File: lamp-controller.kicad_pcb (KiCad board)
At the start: 2 copper layers, 34.9 x 26.5 mm, 33 parts, among them J1 Conn_01x02_Pin, J2 Conn_ARM_JTAG_SWD_10, J3 Conn_01x04_Socket, J4 Conn_01x03_Socket, J5 Conn_01x03_Male, Q1 DMN2053UVT, Q2 DMN2053UVT, SW1 SW_SPST, SW2 SW_Push, U1 MIC5365-3.3YC5, U2 STM32L010F4Px

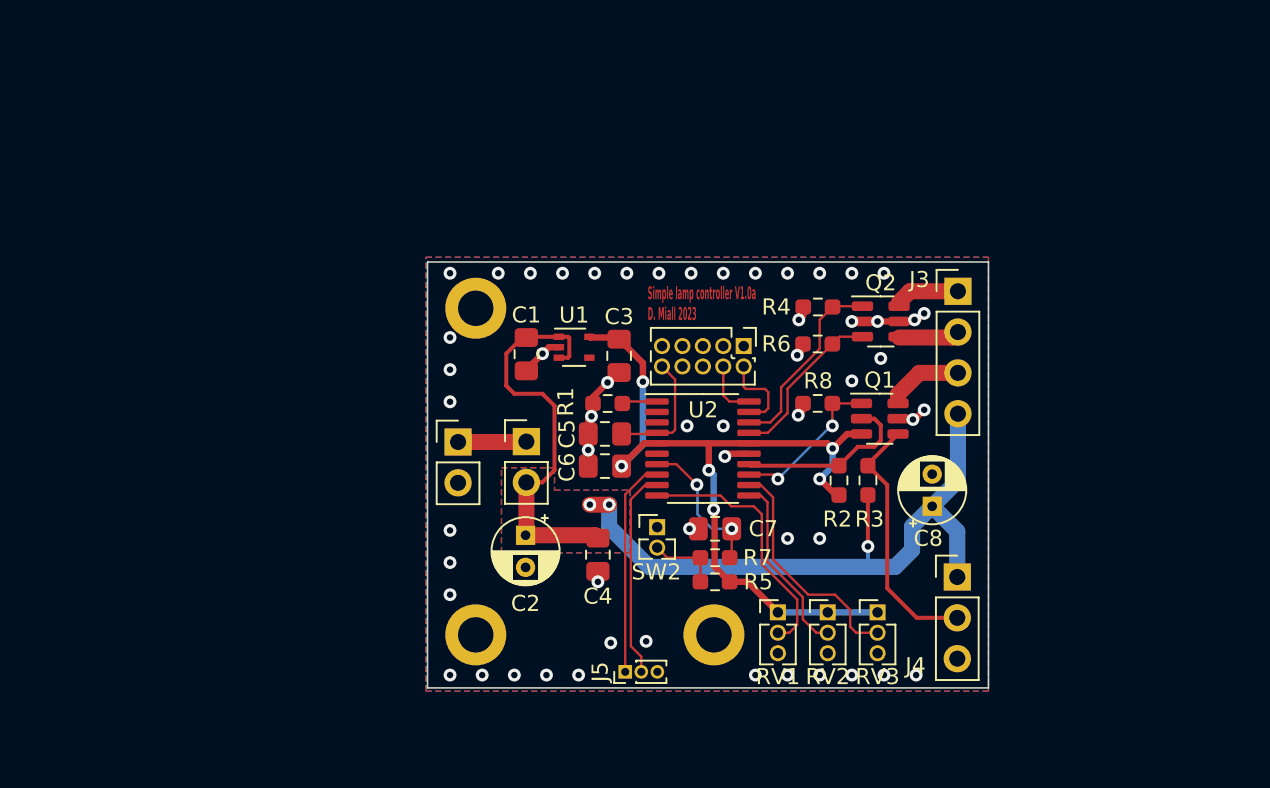
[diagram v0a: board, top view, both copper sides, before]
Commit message: RP2040 Version
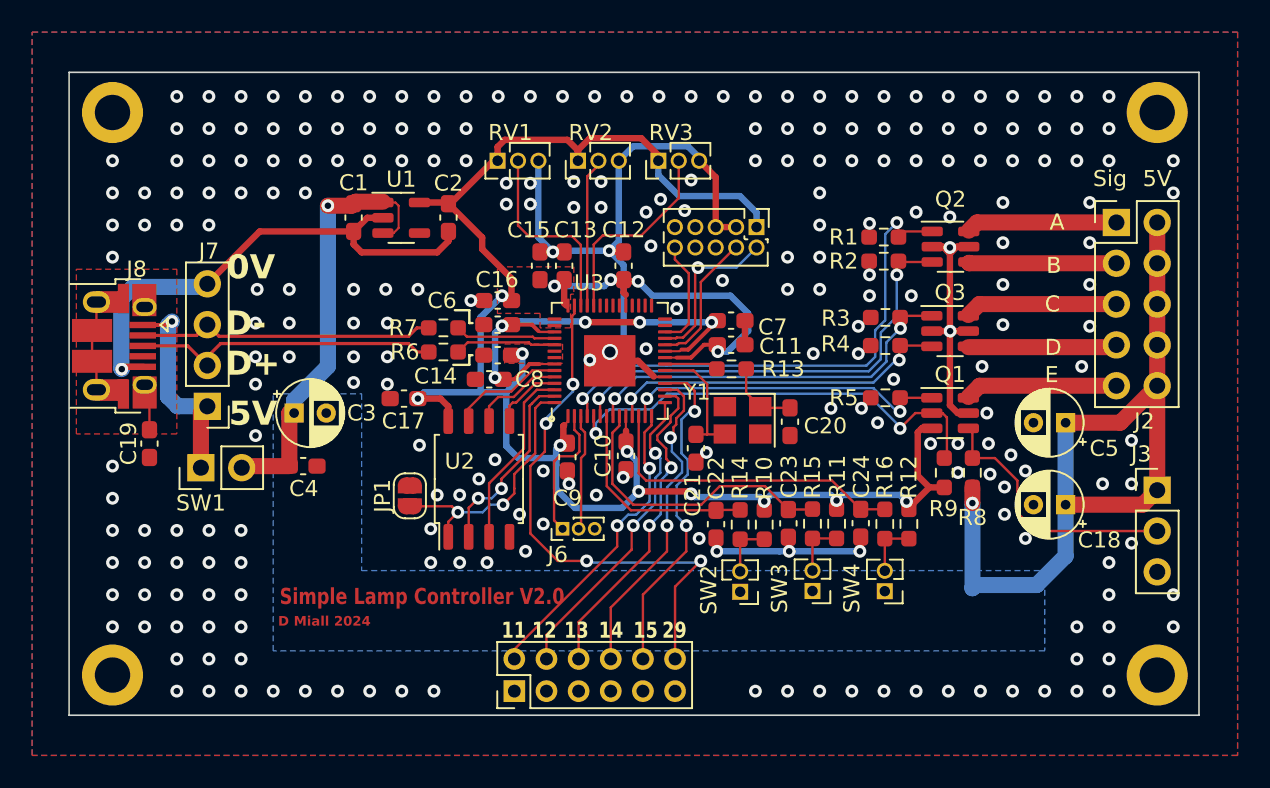
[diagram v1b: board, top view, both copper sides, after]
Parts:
- removed J4: Conn_01x03_Socket, Connector_PinHeader_2.54mm:PinHeader_1x03_P2.54mm_Vertical
- added C10: 100n, Capacitor_SMD:C_0603_1608Metric_Pad1.08x0.95mm_HandSolder, F.Cu at (141.9, 81.4)
- added C11: 100n, Capacitor_SMD:C_0603_1608Metric_Pad1.08x0.95mm_HandSolder, F.Cu at (148.5, 74.5)
- added C12: 100n, Capacitor_SMD:C_0603_1608Metric_Pad1.08x0.95mm_HandSolder, F.Cu at (141.8, 69.5)
- added C13: 100n, Capacitor_SMD:C_0603_1608Metric_Pad1.08x0.95mm_HandSolder, F.Cu at (138.1, 69.5)
- added C14: 100n, Capacitor_SMD:C_0603_1608Metric_Pad1.08x0.95mm_HandSolder, F.Cu at (134.0, 75.1)
- added C15: 100n, Capacitor_SMD:C_0603_1608Metric_Pad1.08x0.95mm_HandSolder, F.Cu at (136.6, 69.5)
- added C16: 100n, Capacitor_SMD:C_0603_1608Metric_Pad1.08x0.95mm_HandSolder, F.Cu at (134.0, 71.7)
- added C17: 0u1, Capacitor_SMD:C_0603_1608Metric_Pad1.08x0.95mm_HandSolder, F.Cu at (128.1, 77.8)
- added C18: 10u 16v, Capacitor_THT:CP_Radial_D4.0mm_P2.00mm, F.Cu at (169.3, 84.4)
- added C19: 10p, Capacitor_SMD:C_0603_1608Metric_Pad1.08x0.95mm_HandSolder, F.Cu at (112.3, 80.6)
- added C20: 27p, Capacitor_SMD:C_0603_1608Metric_Pad1.08x0.95mm_HandSolder, F.Cu at (152.2, 79.2)
- added C21: 27p, Capacitor_SMD:C_0603_1608Metric_Pad1.08x0.95mm_HandSolder, F.Cu at (146.3, 80.9)
- added C22: 0u1, Capacitor_SMD:C_0603_1608Metric_Pad1.08x0.95mm_HandSolder, F.Cu at (147.6, 85.6)
- added C23: 0u1, Capacitor_SMD:C_0603_1608Metric_Pad1.08x0.95mm_HandSolder, F.Cu at (152.1, 85.6)
- added C24: 0u1, Capacitor_SMD:C_0603_1608Metric_Pad1.08x0.95mm_HandSolder, F.Cu at (156.6, 85.5)
- added C9: 100n, Capacitor_SMD:C_0603_1608Metric_Pad1.08x0.95mm_HandSolder, F.Cu at (138.3, 81.4)
- added H4: MountingHole_Pad, MountingHole:MountingHole_2.2mm_M2_DIN965_Pad, F.Cu at (110.0, 95.0)
- added J6: Conn_01x03_Male, Connector_PinHeader_1.00mm:PinHeader_1x03_P1.00mm_Vertical, F.Cu at (138.0, 85.9)
- added J7: Conn_01x04_Socket, Connector_PinHeader_2.54mm:PinHeader_1x04_P2.54mm_Vertical, F.Cu at (115.9, 78.3)
- added J8: USB_B_Micro, Connector_USB:USB_Micro-B_Amphenol_10103594-0001LF_Horizontal, F.Cu at (110.1, 74.5)
- added JP1: SolderJumper_2_Open, Jumper:SolderJumper-2_P1.3mm_Open_RoundedPad1.0x1.5mm, F.Cu at (128.5, 83.8)
- added Q3: DMN2053UVT, Package_TO_SOT_SMD:TSOT-23-6, F.Cu at (162.1, 73.6)
- added R10: 10k, Resistor_SMD:R_0603_1608Metric_Pad0.98x0.95mm_HandSolder, F.Cu at (150.6, 85.6)
- added R11: 10k, Resistor_SMD:R_0603_1608Metric_Pad0.98x0.95mm_HandSolder, F.Cu at (155.1, 85.6)
- added R12: 10k, Resistor_SMD:R_0603_1608Metric_Pad0.98x0.95mm_HandSolder, F.Cu at (159.6, 85.6)
- added R13: 1k3, Resistor_SMD:R_0603_1608Metric_Pad0.98x0.95mm_HandSolder, F.Cu at (148.5, 76.0)
- added R14: 100R, Resistor_SMD:R_0603_1608Metric_Pad0.98x0.95mm_HandSolder, F.Cu at (149.1, 85.6)
- added R15: 100R, Resistor_SMD:R_0603_1608Metric_Pad0.98x0.95mm_HandSolder, F.Cu at (153.6, 85.6)
- added R16: 100R, Resistor_SMD:R_0603_1608Metric_Pad0.98x0.95mm_HandSolder, F.Cu at (158.1, 85.6)
- added R9: 10k, Resistor_SMD:R_0603_1608Metric_Pad0.98x0.95mm_HandSolder, F.Cu at (161.8, 82.4)
- added SW3: SW_Push, Connector_PinHeader_1.27mm:PinHeader_1x02_P1.27mm_Vertical, F.Cu at (153.6, 89.8)
- added SW4: SW_Push, Connector_PinHeader_1.27mm:PinHeader_1x02_P1.27mm_Vertical, F.Cu at (158.1, 89.8)
- added U3: RP2040, Package_DFN_QFN:QFN-56-1EP_7x7mm_P0.4mm_EP3.2x3.2mm, F.Cu at (140.9, 75.5)
- added Y1: RH100-12.000-18-2030-TR, Crystal:Crystal_SMD_3225-4Pin_3.2x2.5mm, F.Cu at (149.2, 79.2)
- C1, C4: footprint Capacitor_SMD:C_0805_2012Metric_Pad1.18x1.45mm_HandSolder -> Capacitor_SMD:C_0603_1608Metric_Pad1.08x0.95mm_HandSolder
- C2: value 10u 16v -> 1u; footprint Capacitor_THT:CP_Radial_D4.0mm_P2.00mm -> Capacitor_SMD:C_0603_1608Metric_Pad1.08x0.95mm_HandSolder
- C3: value 1u -> 10u 16v; footprint Capacitor_SMD:C_0805_2012Metric_Pad1.18x1.45mm_HandSolder -> Capacitor_THT:CP_Radial_D4.0mm_P2.00mm
- C5: value 0u1 -> 10u 16v; footprint Capacitor_SMD:C_0805_2012Metric_Pad1.18x1.45mm_HandSolder -> Capacitor_THT:CP_Radial_D4.0mm_P2.00mm
- C6, C7: value 0u1 -> 100n; footprint Capacitor_SMD:C_0805_2012Metric_Pad1.18x1.45mm_HandSolder -> Capacitor_SMD:C_0603_1608Metric_Pad1.08x0.95mm_HandSolder
- C8: value 10u 16v -> 100n; footprint Capacitor_THT:CP_Radial_D4.0mm_P2.00mm -> Capacitor_SMD:C_0603_1608Metric_Pad1.08x0.95mm_HandSolder
- J1: value Conn_01x02_Pin -> Conn_02x06_Odd_Even; footprint Connector_PinHeader_2.54mm:PinHeader_1x02_P2.54mm_Vertical -> Connector_PinHeader_2.00mm:PinHeader_2x06_P2.00mm_Vertical
- J2: value Conn_ARM_JTAG_SWD_10 -> Conn_02x05_Odd_Even; footprint Connector_PinHeader_1.27mm:PinHeader_2x05_P1.27mm_Vertical -> Connector_PinHeader_2.54mm:PinHeader_2x05_P2.54mm_Vertical
- J3: value Conn_01x04_Socket -> Conn_01x03_Socket; footprint Connector_PinHeader_2.54mm:PinHeader_1x04_P2.54mm_Vertical -> Connector_PinHeader_2.54mm:PinHeader_1x03_P2.54mm_Vertical
- J5: value Conn_01x03_Male -> Conn_ARM_JTAG_SWD_10; footprint Connector_PinHeader_1.00mm:PinHeader_1x03_P1.00mm_Vertical -> Connector_PinHeader_1.27mm:PinHeader_2x05_P1.27mm_Vertical
- R6: value 10k -> 27R
- R7: value 100R -> 27R
- U1: value MIC5365-3.3YC5 -> AP2202K-3.3TRG1; footprint Package_TO_SOT_SMD:SOT-353_SC-70-5 -> Package_TO_SOT_SMD:SOT-23-5
- U2: value STM32L010F4Px -> W25Q16JVSS; footprint Package_SO:TSSOP-20_4.4x6.5mm_P0.65mm -> Package_SO:SOIC-8_5.275x5.275mm_P1.27mm
- moved H2 53.4 mm to (175.0, 60.0)
- moved RV1 33.1 mm to (134.0, 63.0), turned to 90 degrees
- moved RV2 32.1 mm to (139.0, 63.0), turned to 90 degrees
- moved RV3 31.2 mm to (144.0, 63.0), turned to 90 degrees
- moved J5 28.9 mm to (150.1, 67.1), turned to -90 degrees
- moved C8 28.7 mm to (133.4, 76.6), turned to 0 degrees
- moved C5 28.7 mm to (169.3, 79.3)
- moved H3 27.7 mm to (175.0, 95.0)
- moved H1 25.7 mm to (110.0, 60.0)
- moved J2 24.4 mm to (172.5, 66.8), turned to 0 degrees
- moved R6 23.3 mm to (130.6, 74.9), turned to 0 degrees
- moved R7 22.1 mm to (130.6, 73.4)
- moved C3 20.5 mm to (121.3, 78.7), turned to 0 degrees
- moved C2 20.3 mm to (130.9, 66.5)
- moved SW1 20.3 mm to (115.5, 82.1), turned to 90 degrees
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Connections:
- C2 pad 1: +5V -> +3V3
- C3 pad 1: +3V3 -> +5V
- C5 pad 1: /rst -> +5V
- C6 pad 1: +3V3 -> GND
- C6 pad 2: GND -> +1V1
- C7 pad 1: /Button -> GND
- C7 pad 2: GND -> +1V1
- C8 pad 1: +5V -> GND
- C8 pad 2: GND -> +1V1
- J1 pad 1: /5Vin -> GND
- J1 pad 2: GND -> Net-(J1-Pin_2)
- J2 pad 1: /3v3 -> /A_o
- J2 pad 10: /rst -> +5V
- J2 pad 2: /swdio -> +5V
- J2 pad 3: GND -> /B_o
- J2 pad 4: /swclk -> +5V
- J2 pad 5: GND -> /C_o
- J2 pad 6: unconnected-(J2-SWO/TDO-Pad6) -> +5V
- J2 pad 7: unconnected-(J2-KEY-Pad7) -> /D_o
- J2 pad 8: unconnected-(J2-NC/TDI-Pad8) -> +5V
- J2 pad 9: unconnected-(J2-GNDDetect-Pad9) -> /E_o
- J3 pad 1: /A_o -> +5V
- J3 pad 2: /B_o -> /PxCtrl
- J3 pad 3: /C_o -> GND
- J5 pad 1: /LPUART1_TX -> +3V3
- J5 pad 2: /LPUART1_RX -> /swdio
- Q1 pad 1: /C -> /E
- Q1 pad 6: /C_o -> /E_o
- R1 pad 1: Net-(U2-PB9) -> /A
- R2 pad 1: +3V3 -> /B
- R2 pad 2: /PxCtrlLv -> GND
- R3 pad 1: +5V -> /C
- R3 pad 2: /PxCtrl -> GND
- R4 pad 1: /A -> /D
- R5 pad 1: +3V3 -> /E
- R5 pad 2: Net-(R5-Pad2) -> GND
- R6 pad 1: /B -> /USB_D+
- R6 pad 2: GND -> Net-(U3-USB_DP)
- R7 pad 1: Net-(R5-Pad2) -> /USB_D-
- R7 pad 2: /Button -> Net-(U3-USB_DM)
- R8 pad 1: /C -> +5V
- R8 pad 2: GND -> /PxCtrl
- RV1 pad 2: /A_Pot -> /Pot_3
- RV2 pad 2: /B_Pot -> /Pot_2
- RV3 pad 2: /C_Pot -> /Pot_1
- SW2 pad 2: Net-(R5-Pad2) -> Net-(R10-Pad2)
- U2 pad 1: Net-(U2-PB9) -> /SSel
- U2 pad 2: unconnected-(U2-PC14-Pad2) -> /SD1
- U2 pad 3: unconnected-(U2-PC15-Pad3) -> /SD2
- U2 pad 4: /rst -> GND
- U2 pad 5: +3V3 -> /SD0
- U2 pad 6: unconnected-(U2-PA0-Pad6) -> /SCLK
- U2 pad 7: /Button -> /SD3
- U2 pad 8: /LPUART1_TX -> +3V3
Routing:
- net GND: track 23.2 -> 103.9 mm, vias 55 -> 250
- net +3V3: track 50.0 -> 130.6 mm, vias 6 -> 14
- net /ADC3: track 0.00 -> 33.5 mm, vias 0 -> 4
- net +1V1: track 0.00 -> 28.6 mm, vias 0 -> 5
- net /D: track 0.00 -> 21.7 mm, vias 0 -> 2
- net Net-(J1-Pin_10): track 0.00 -> 21.1 mm, vias 0 -> 2
- net /A: track 12.0 -> 32.6 mm, vias 0 -> 2
- net /E: track 0.00 -> 20.6 mm, vias 0 -> 2
- net Net-(J1-Pin_6): track 0.00 -> 20.4 mm, vias 0 -> 2
- net Net-(J1-Pin_8): track 0.00 -> 20.2 mm, vias 0 -> 2
- net /Button_3: track 0.00 -> 19.8 mm
- net Net-(J1-Pin_4): track 0.00 -> 19.5 mm, vias 0 -> 2
- net /USB_D+: track 0.00 -> 19.4 mm
- net Net-(J1-Pin_2): track 0.00 -> 19.2 mm, vias 0 -> 2
- net /USB_D-: track 0.00 -> 18.6 mm
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- added copper zone on F.Cu, net +3V3
- added copper zone on F.Cu, net Net-(J8-Shield)
- removed copper zone on F.Cu, net +5V
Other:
- board size 34.9 x 26.5 mm -> 70.3 x 40 mm
- board text added: "0V"
- board text added: "11"
- board text added: "12"
- board text added: "13"
- board text added: "14"
- board text added: "15"
- board text added: "29"
- board text added: "5V"
- board text added: "A"
- board text added: "B"
- board text added: "C"
- board text added: "D"
- board text added: "D Miall 2024"
- board text added: "D+"
- board text added: "D-"
- board text added: "E"
- board text added: "Sig"
- board text added: "Simple Lamp Controller V2.0"
- board text removed: "Simple lamp controller V1.0a D. Miall 2023"
